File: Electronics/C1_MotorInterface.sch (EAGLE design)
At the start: 19 parts, among them IC1 ACS750LCA-050, J1 PIN1-2, J2 PIN1-2, J3 PIN1-2, J4 PIN1-2, J5 PIN1-2, J6 PIN1-2, J7 PIN1-2, J8 PIN1-2, K1 30A 120V

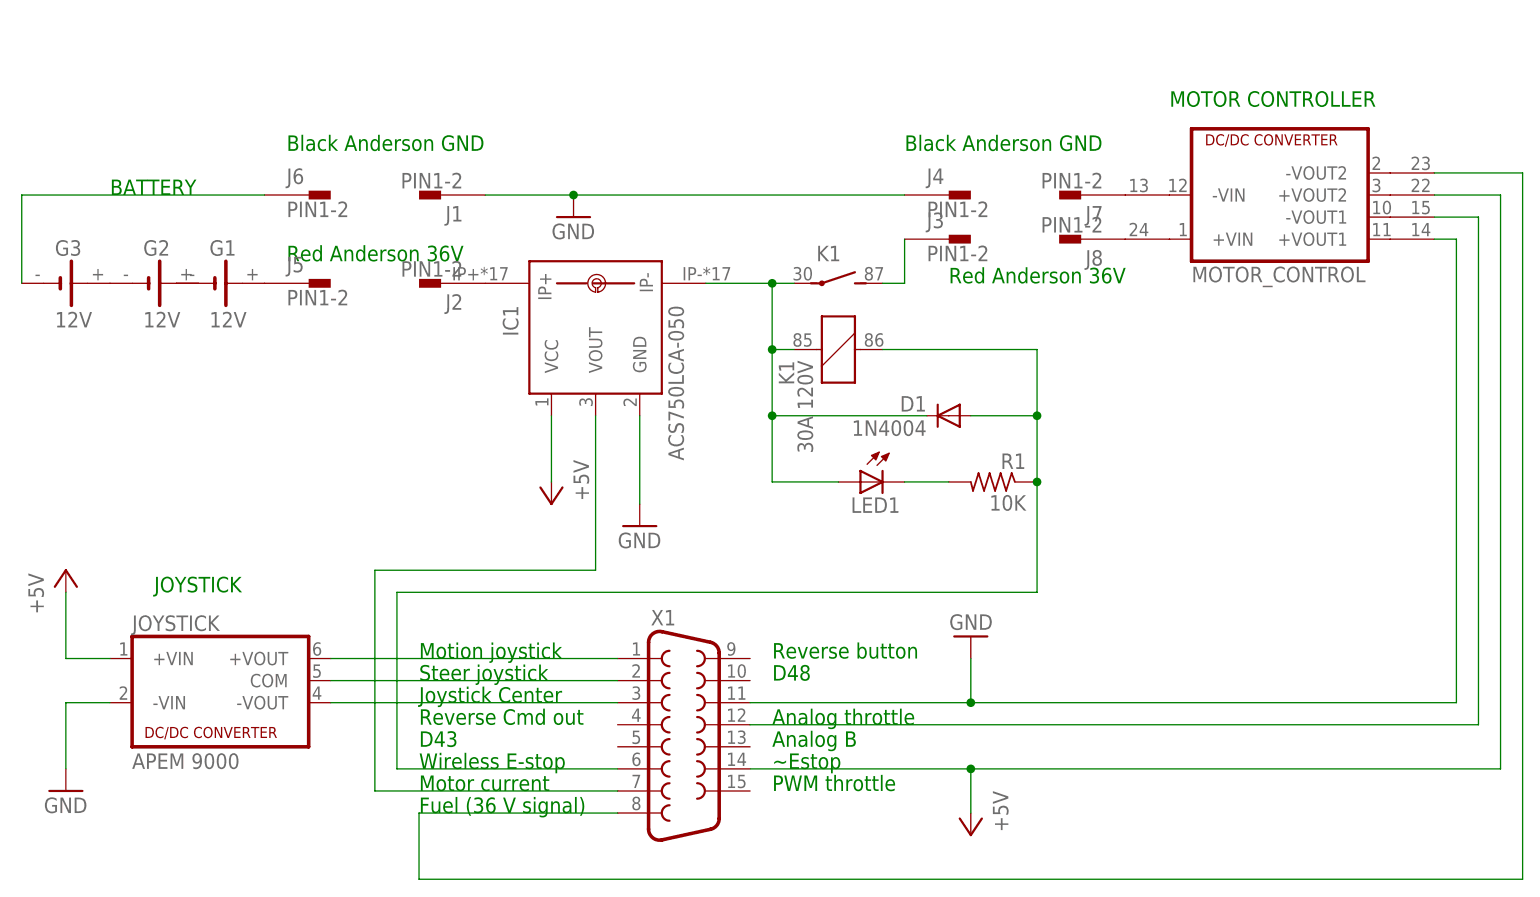
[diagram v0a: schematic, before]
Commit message: update to Sourceforge 123
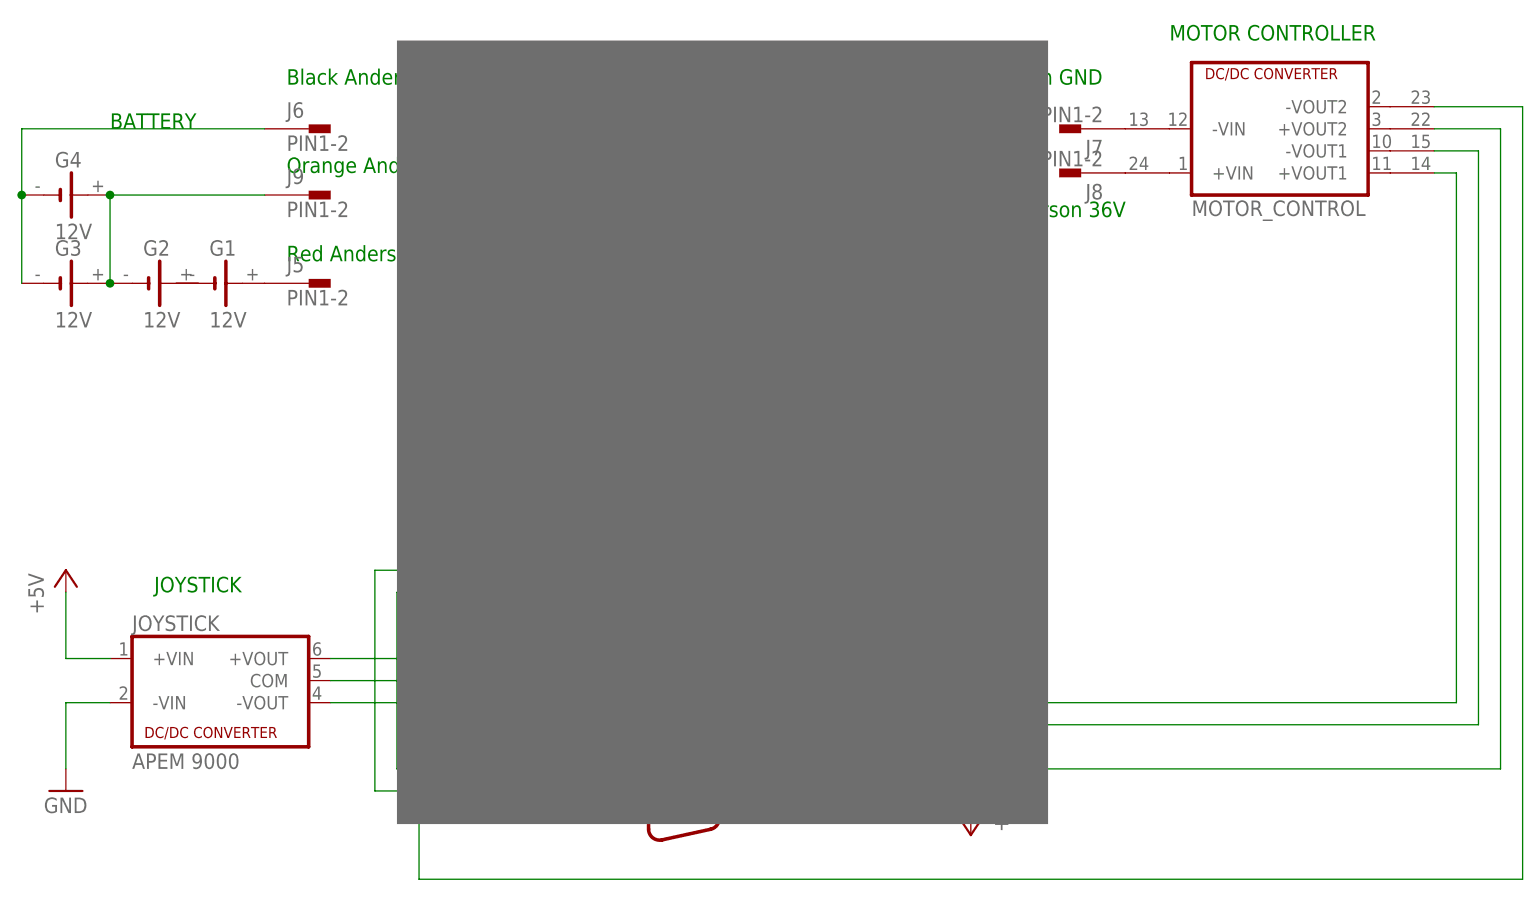
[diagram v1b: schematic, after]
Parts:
- added G4: 12V, battery:SL-150-1/2AA/PR
- added J10, J9: PIN1-2, con-faston:PIN1-2
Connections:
- new net N$16: IC1.IP-, K12.P
- net N$1: now also J10.1; no longer IC1.IP-, K12.P
- net N$7: now also G4.+, J9.1
- net N$8: now also G4.-, J6.1
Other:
- note added: "Normally closed"
- note added: "Orange Anderson 12V"
- moved on the sheet: J1, J3, J4, J6, J7, J8, MOTOR_CONTROL
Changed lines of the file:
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@@
 <part name="P+3" library="supply1" deviceset="+5V" device=""/>
 <part name="GND4" library="supply1" deviceset="GND" device=""/>
+<part name="G4" library="battery" deviceset="SL-150-1/2AA/PR" device="" value="12V"/>
+<part name="J9" library="con-faston" deviceset="PIN1-2" device=""/>
+<part name="J10" library="con-faston" deviceset="PIN1-2" device=""/>
 </parts>
 <sheets>
@@
 <text x="48.26" y="2.54" size="1.778" layer="91">PWM throttle</text>
 <text x="-7.62" y="63.5" size="1.778" layer="91">Red Anderson 36V</text>
-<text x="68.58" y="60.96" size="1.778" layer="91">Red Anderson 36V</text>
-<text x="-7.62" y="76.2" size="1.778" layer="91">Black Anderson GND</text>
-<text x="63.5" y="76.2" size="1.778" layer="91">Black Anderson GND</text>
+<text x="68.58" y="68.58" size="1.778" layer="91">Red Anderson 36V</text>
+<text x="-7.62" y="83.82" size="1.778" layer="91">Black Anderson GND</text>
+<text x="63.5" y="83.82" size="1.778" layer="91">Black Anderson GND</text>
 <text x="-22.86" y="25.4" size="1.778" layer="91">JOYSTICK</text>
-<text x="93.98" y="81.28" size="1.778" layer="91">MOTOR CONTROLLER</text>
-<text x="-27.94" y="71.12" size="1.778" layer="91">BATTERY</text>
+<text x="93.98" y="88.9" size="1.778" layer="91">MOTOR CONTROLLER</text>
+<text x="-27.94" y="78.74" size="1.778" layer="91">BATTERY</text>
+<text x="50.8" y="58.42" size="1.778" layer="91">Normally closed</text>
+<rectangle x1="5.08" y1="-1.27" x2="80.01" y2="88.9" layer="95"/>
+<text x="-7.62" y="73.66" size="1.778" layer="91">Orange Anderson 12V</text>
 </plain>
 <instances>
@@
 <instance part="GND1" gate="1" x="71.12" y="20.32" rot="R180"/>
 <instance part="P+1" gate="1" x="71.12" y="-2.54" rot="R180"/>
-<instance part="J1" gate="G$1" x="10.16" y="71.12" rot="R180"/>
+<instance part="J1" gate="G$1" x="10.16" y="78.74" rot="R180"/>
 <instance part="J2" gate="G$1" x="10.16" y="60.96" rot="R180"/>
-<instance part="J3" gate="G$1" x="68.58" y="66.04"/>
-<instance part="J4" gate="G$1" x="68.58" y="71.12"/>
+<instance part="J3" gate="G$1" x="68.58" y="73.66"/>
+<instance part="J4" gate="G$1" x="68.58" y="78.74"/>
 <instance part="K1" gate="1" x="55.88" y="53.34" rot="MR270"/>
 <instance part="K1" gate="2" x="55.88" y="60.96" rot="R270"/>
@@
 <instance part="LED1" gate="G$1" x="58.42" y="38.1" rot="MR270"/>
 <instance part="R1" gate="G$1" x="73.66" y="38.1" rot="MR0"/>
-<instance part="GND2" gate="1" x="25.4" y="68.58"/>
+<instance part="GND2" gate="1" x="25.4" y="76.2"/>
 <instance part="G1" gate="G$1" x="-15.24" y="60.96"/>
 <instance part="G2" gate="G$1" x="-22.86" y="60.96"/>
 <instance part="G3" gate="G$1" x="-33.02" y="60.96"/>
 <instance part="J5" gate="G$1" x="-5.08" y="60.96"/>
-<instance part="J6" gate="G$1" x="-5.08" y="71.12"/>
-<instance part="MOTOR_CONTROL" gate="G$1" x="106.68" y="68.58" rot="MR180"/>
-<instance part="J7" gate="G$1" x="83.82" y="71.12" rot="R180"/>
-<instance part="J8" gate="G$1" x="83.82" y="66.04" rot="R180"/>
+<instance part="J6" gate="G$1" x="-5.08" y="78.74"/>
+<instance part="MOTOR_CONTROL" gate="G$1" x="106.68" y="76.2" rot="MR180"/>
+<instance part="J7" gate="G$1" x="83.82" y="78.74" rot="R180"/>
+<instance part="J8" gate="G$1" x="83.82" y="73.66" rot="R180"/>
 <instance part="IC1" gate="G$1" x="27.94" y="55.88" rot="MR270"/>
 <instance part="GND3" gate="1" x="33.02" y="33.02"/>
@@
 <instance part="P+3" gate="1" x="-33.02" y="27.94"/>
 <instance part="GND4" gate="1" x="-33.02" y="2.54"/>
+<instance part="G4" gate="G$1" x="-33.02" y="71.12"/>
+<instance part="J9" gate="G$1" x="-5.08" y="71.12"/>
+<instance part="J10" gate="G$1" x="10.16" y="71.12" rot="R180"/>
 </instances>
 <busses>
@@
 <wire x1="71.12" y1="12.7" x2="71.12" y2="17.78" width="0.1524" layer="91"/>
 <junction x="71.12" y="12.7"/>
-<wire x1="127" y1="66.04" x2="127" y2="12.7" width="0.1524" layer="91"/>
+<wire x1="127" y1="73.66" x2="127" y2="12.7" width="0.1524" layer="91"/>
 <wire x1="127" y1="12.7" x2="71.12" y2="12.7" width="0.1524" layer="91"/>
 <pinref part="MOTOR_CONTROL" gate="G$1" pin="+VOUT@1"/>
-<wire x1="124.46" y1="66.04" x2="127" y2="66.04" width="0.1524" layer="91"/>
+<wire x1="124.46" y1="73.66" x2="127" y2="73.66" width="0.1524" layer="91"/>
 </segment>
 <segment>
 <pinref part="J1" gate="G$1" pin="1"/>
 <pinref part="J4" gate="G$1" pin="1"/>
-<wire x1="15.24" y1="71.12" x2="25.4" y2="71.12" width="0.1524" layer="91"/>
+<wire x1="15.24" y1="78.74" x2="25.4" y2="78.74" width="0.1524" layer="91"/>
 <pinref part="GND2" gate="1" pin="GND"/>
-<wire x1="25.4" y1="71.12" x2="63.5" y2="71.12" width="0.1524" layer="91"/>
-<junction x="25.4" y="71.12"/>
+<wire x1="25.4" y1="78.74" x2="63.5" y2="78.74" width="0.1524" layer="91"/>
+<junction x="25.4" y="78.74"/>
 </segment>
 <segment>
@@
 <pinref part="P+1" gate="1" pin="+5V"/>
 <pinref part="MOTOR_CONTROL" gate="G$1" pin="+VOUT@2"/>
-<wire x1="124.46" y1="71.12" x2="132.08" y2="71.12" width="0.1524" layer="91"/>
-<wire x1="132.08" y1="71.12" x2="132.08" y2="5.08" width="0.1524" layer="91"/>
+<wire x1="124.46" y1="78.74" x2="132.08" y2="78.74" width="0.1524" layer="91"/>
+<wire x1="132.08" y1="78.74" x2="132.08" y2="5.08" width="0.1524" layer="91"/>
 <wire x1="132.08" y1="5.08" x2="71.12" y2="5.08" width="0.1524" layer="91"/>
 <wire x1="71.12" y1="5.08" x2="71.12" y2="0" width="0.1524" layer="91"/>
@@
 <net name="N$1" class="0">
 <segment>
-<pinref part="K1" gate="2" pin="P"/>
-<wire x1="48.26" y1="60.96" x2="50.8" y2="60.96" width="0.1524" layer="91"/>
 <pinref part="K1" gate="1" pin="1"/>
 <wire x1="50.8" y1="53.34" x2="48.26" y2="53.34" width="0.1524" layer="91"/>
-<wire x1="48.26" y1="60.96" x2="48.26" y2="53.34" width="0.1524" layer="91"/>
-<junction x="48.26" y="53.34"/>
 <pinref part="D1" gate="1" pin="C"/>
 <wire x1="66.04" y1="45.72" x2="48.26" y2="45.72" width="0.1524" layer="91"/>
@@
 <wire x1="48.26" y1="38.1" x2="48.26" y2="45.72" width="0.1524" layer="91"/>
 <junction x="48.26" y="45.72"/>
-<pinref part="IC1" gate="G$1" pin="IP-"/>
-<wire x1="40.64" y1="60.96" x2="48.26" y2="60.96" width="0.1524" layer="91"/>
-<junction x="48.26" y="60.96"/>
+<pinref part="J10" gate="G$1" pin="1"/>
+<wire x1="15.24" y1="71.12" x2="48.26" y2="71.12" width="0.1524" layer="91"/>
+<wire x1="48.26" y1="71.12" x2="48.26" y2="53.34" width="0.1524" layer="91"/>
+<junction x="48.26" y="53.34"/>
 </segment>
 </net>
@@
 <pinref part="G2" gate="G$1" pin="-"/>
 <pinref part="G3" gate="G$1" pin="+"/>
+<wire x1="-27.94" y1="60.96" x2="-27.94" y2="71.12" width="0.1524" layer="91"/>
+<wire x1="-27.94" y1="71.12" x2="-10.16" y2="71.12" width="0.1524" layer="91"/>
+<pinref part="G4" gate="G$1" pin="+"/>
+<junction x="-27.94" y="71.12"/>
+<pinref part="J9" gate="G$1" pin="1"/>
+<junction x="-27.94" y="60.96"/>
 </segment>
 </net>
@@
 <pinref part="G3" gate="G$1" pin="-"/>
 <wire x1="-38.1" y1="60.96" x2="-38.1" y2="71.12" width="0.1524" layer="91"/>
-<wire x1="-38.1" y1="71.12" x2="-10.16" y2="71.12" width="0.1524" layer="91"/>
+<wire x1="-38.1" y1="71.12" x2="-38.1" y2="78.74" width="0.1524" layer="91"/>
+<wire x1="-38.1" y1="78.74" x2="-10.16" y2="78.74" width="0.1524" layer="91"/>
+<pinref part="J6" gate="G$1" pin="1"/>
+<pinref part="G4" gate="G$1" pin="-"/>
+<junction x="-38.1" y="71.12"/>
 </segment>
 </net>
@@
 <wire x1="7.62" y1="0" x2="7.62" y2="-7.62" width="0.1524" layer="91"/>
 <wire x1="7.62" y1="-7.62" x2="134.62" y2="-7.62" width="0.1524" layer="91"/>
-<wire x1="134.62" y1="-7.62" x2="134.62" y2="73.66" width="0.1524" layer="91"/>
+<wire x1="134.62" y1="-7.62" x2="134.62" y2="81.28" width="0.1524" layer="91"/>
 <pinref part="MOTOR_CONTROL" gate="G$1" pin="-VOUT@2"/>
-<wire x1="124.46" y1="73.66" x2="134.62" y2="73.66" width="0.1524" layer="91"/>
+<wire x1="124.46" y1="81.28" x2="134.62" y2="81.28" width="0.1524" layer="91"/>
 </segment>
 </net>
@@
 <pinref part="J3" gate="G$1" pin="1"/>
 <wire x1="60.96" y1="60.96" x2="63.5" y2="60.96" width="0.1524" layer="91"/>
-<wire x1="63.5" y1="60.96" x2="63.5" y2="66.04" width="0.1524" layer="91"/>
+<wire x1="63.5" y1="60.96" x2="63.5" y2="73.66" width="0.1524" layer="91"/>
 </segment>
 </net>
@@
 <pinref part="X1" gate="-1" pin="12"/>
 <wire x1="45.72" y1="10.16" x2="129.54" y2="10.16" width="0.1524" layer="91"/>
-<wire x1="129.54" y1="10.16" x2="129.54" y2="68.58" width="0.1524" layer="91"/>
+<wire x1="129.54" y1="10.16" x2="129.54" y2="76.2" width="0.1524" layer="91"/>
 <pinref part="MOTOR_CONTROL" gate="G$1" pin="-VOUT@1"/>
-<wire x1="129.54" y1="68.58" x2="124.46" y2="68.58" width="0.1524" layer="91"/>
+<wire x1="129.54" y1="76.2" x2="124.46" y2="76.2" width="0.1524" layer="91"/>
 </segment>
 </net>
@@
 </segment>
 </net>
+<net name="N$16" class="0">
+<segment>
+<pinref part="K1" gate="2" pin="P"/>
+<pinref part="IC1" gate="G$1" pin="IP-"/>
+<wire x1="40.64" y1="60.96" x2="50.8" y2="60.96" width="0.1524" layer="91"/>
+</segment>
+</net>
